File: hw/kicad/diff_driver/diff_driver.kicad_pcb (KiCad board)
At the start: 2 copper layers, 32 x 22 mm, 14 parts, among them J1 CONN_01X07, J2 RJ45_LED, U1 am26ls31, U2 HT75XX-1

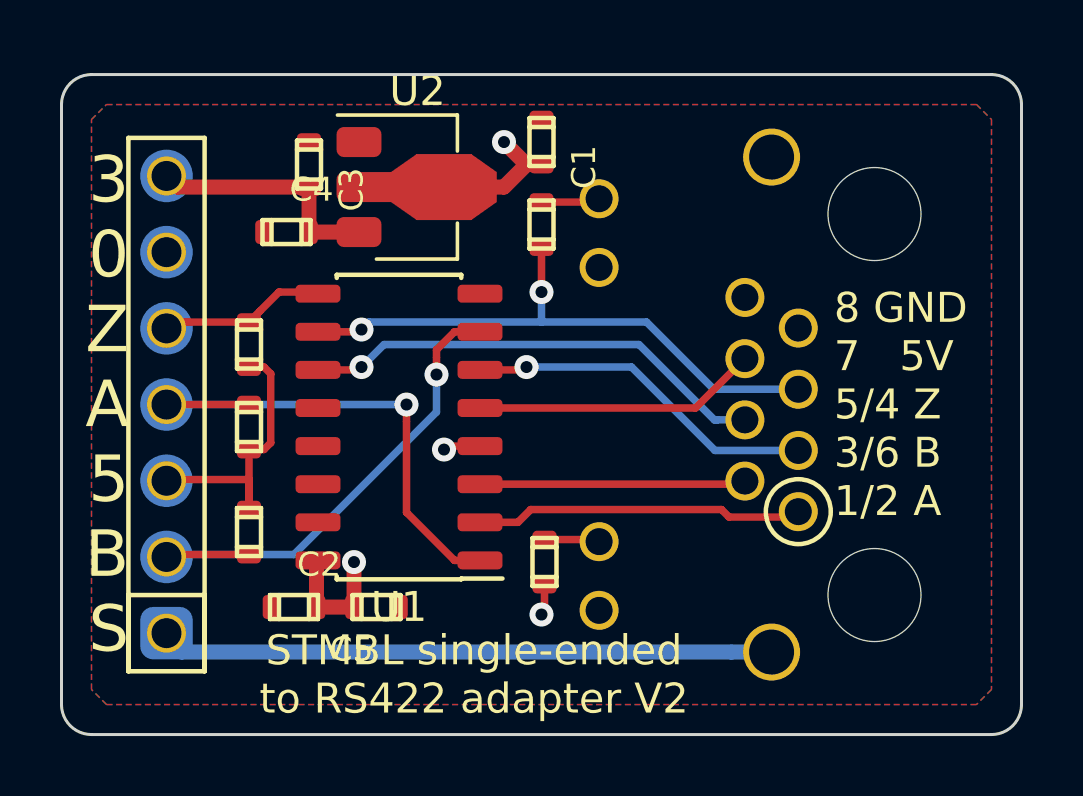
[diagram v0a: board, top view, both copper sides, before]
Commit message: added HW files
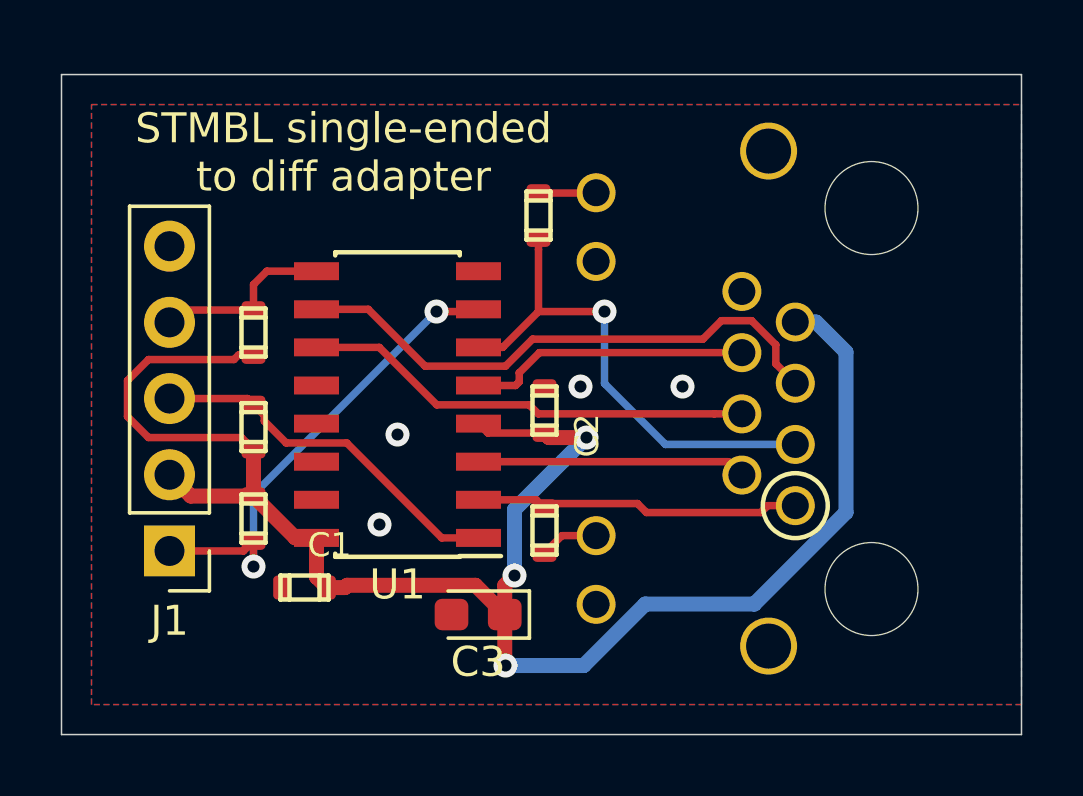
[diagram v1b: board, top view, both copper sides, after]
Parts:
- removed C4, C5: 1n, stmbl:C_0603
- removed U2: HT75XX-1, stmbl:SOT-89-3
- C1, C2: value 100n -> C
- C3: value 100n -> CP; footprint stmbl:C_0603 -> Capacitor_Tantalum_SMD:CP_EIA-2012-15_AVX-P
- J1: value CONN_01X07 -> CONN_01X05; footprint stmbl:Pin_Header_RM2.54_1x7_UP -> Connector_PinHeader_2.54mm:PinHeader_1x05_P2.54mm_Vertical
- R1, R2, R3: value 3.9k -> R
- R4, R5: value 560 -> R
- U1: value am26ls31 -> LTC1688; footprint stmbl:SOIC-16 -> Package_SO:SOIC-16_3.9x9.9mm_P1.27mm
- moved C1 16.8 mm to (151.1, 97.1), turned to 180 degrees
- moved C3 16.0 mm to (156.9, 98.0), turned to 180 degrees
- moved C2 10.6 mm to (159.1, 91.2), turned to 90 degrees
- moved J1 2.74 mm to (146.6, 95.9)
- moved R4 1.05 mm to (159.1, 95.2), turned to 270 degrees
- moved U1 0.75 mm to (154.2, 91.0)
- moved R2 0.47 mm to (149.4, 94.8)
- moved R3 0.43 mm to (149.4, 88.6)
- moved R5 0.32 mm to (158.9, 84.7)
- moved J2 0.22 mm to (175.4, 90.8)
- moved R1 0.15 mm to (149.4, 91.8)
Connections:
- C3 pad 1: +3V3 -> +5V
- J1 pad 1: GNDA -> B
- J1 pad 2: B -> +5V
- J1 pad 3: +5V -> A
- J1 pad 4: A -> IDX
- J1 pad 5: IDX -> GND
- R4 pad 1: +5V -> Net-(J2-Pad1)
- R5 pad 1: Net-(J2-Pad5) -> Net-(J2-Pad3)
- U1 pad 13: (no net) -> Net-(U1-Pad13)
- U1 pad 14: (no net) -> Net-(U1-Pad14)
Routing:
- net +5V: track 24.2 -> 59.4 mm, vias 4 -> 3
- net GNDA: track 20.5 -> 0.00 mm
- net +3V3: track 8.07 -> 0.00 mm
- net A: track 17.5 -> 12.3 mm, vias 1 -> 0
- net Net-(J2-Pad3): track 11.8 -> 16.7 mm
- net B: track 17.6 -> 16.2 mm, vias 1 -> 2
- net Net-(J2-Pad5): track 19.6 -> 18.6 mm, vias 2 -> 0
- net IDX: track 5.57 -> 6.10 mm
- net Net-(J2-Pad4): track 15.6 -> 15.1 mm, vias 1 -> 0
- net GND: vias 0 -> 4
- added copper zone on B.Cu, net GND
- removed copper zone on B.Cu, net +5V
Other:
- outline, holes or cut-outs redrawn
- board text added: "5V"
- board text added: "A/U"
- board text added: "B/V"
- board text added: "GND"
- board text added: "IDX/W"
- board text added: "STMBL single-ended to diff adapter"
- board text removed: "3 0 Z A 5 B S"
- board text removed: "3.3V GND Z/W A/U 5V B/V SHIELD"
- board text removed: "8 GND 7 5V 5/4 Z 3/6 B 1/2 A"
- board text removed: "STMBL single-ended to RS422 adapter V2"
